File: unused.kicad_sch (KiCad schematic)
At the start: 7 parts, among them J6 FPGA GPIO, J7 FPGA_B3_GPIO, U8 T20Q144xx

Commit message: Added Manufacturer + Part info for most components.
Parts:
- C11, C14, C74, C75: Manufacturer (none) -> Samsung; Part (none) -> CL10B104KB8NFN
- J6: Manufacturer (none) -> Adam Tech; Part (none) -> PH2-20-UA
- J7: Manufacturer (none) -> Adam Tech; Part (none) -> PH2-08-UA
- U8: Manufacturer (none) -> Efinix; Part (none) -> T20Q144C4
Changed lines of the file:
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@@
+      (effects (font (size 1.27 1.27)) hide)
+    )
+    (property "Manufacturer" "Samsung" (at 88.9 97.79 0)
+      (effects (font (size 1.27 1.27)) hide)
+    )
+    (property "Part" "CL10B104KB8NFN" (at 88.9 97.79 0)
       (effects (font (size 1.27 1.27)) hide)
     )
@@
     )
     (property "Datasheet" "~" (at 86.36 173.99 0)
+      (effects (font (size 1.27 1.27)) hide)
+    )
+    (property "Manufacturer" "Adam Tech" (at 86.36 173.99 0)
+      (effects (font (size 1.27 1.27)) hide)
+    )
+    (property "Part" "PH2-08-UA" (at 86.36 173.99 0)
       (effects (font (size 1.27 1.27)) hide)
     )
@@
       (effects (font (size 1.27 1.27)) hide)
     )
+    (property "Manufacturer" "Samsung" (at 127 63.5 0)
+      (effects (font (size 1.27 1.27)) hide)
+    )
+    (property "Part" "CL10B104KB8NFN" (at 127 63.5 0)
+      (effects (font (size 1.27 1.27)) hide)
+    )
     (pin "1")
     (pin "2")
@@
     )
     (property "Datasheet" "~" (at 85.725 137.16 0)
+      (effects (font (size 1.27 1.27)) hide)
+    )
+    (property "Manufacturer" "Adam Tech" (at 85.725 137.16 0)
+      (effects (font (size 1.27 1.27)) hide)
+    )
+    (property "Part" "PH2-20-UA" (at 85.725 137.16 0)
       (effects (font (size 1.27 1.27)) hide)
     )
@@
     )
     (property "Datasheet" "https://www.efinixinc.com/docs/trion8-ds-v4.4.pdf" (at 194.31 152.4 0)
+      (effects (font (size 1.27 1.27)) hide)
+    )
+    (property "Manufacturer" "Efinix" (at 194.31 125.73 0)
+      (effects (font (size 1.27 1.27)) hide)
+    )
+    (property "Part" "T20Q144C4" (at 194.31 125.73 0)
       (effects (font (size 1.27 1.27)) hide)
     )
@@
       (effects (font (size 1.27 1.27)) hide)
     )
+    (property "Manufacturer" "Efinix" (at 191.77 76.2 0)
+      (effects (font (size 1.27 1.27)) hide)
+    )
+    (property "Part" "T20Q144C4" (at 191.77 76.2 0)
+      (effects (font (size 1.27 1.27)) hide)
+    )
     (pin "76")
     (pin "141")
@@
       (effects (font (size 1.27 1.27)) hide)
     )
+    (property "Manufacturer" "Samsung" (at 127 97.79 0)
+      (effects (font (size 1.27 1.27)) hide)
+    )
+    (property "Part" "CL10B104KB8NFN" (at 127 97.79 0)
+      (effects (font (size 1.27 1.27)) hide)
+    )
     (pin "1")
     (pin "2")
@@
       (effects (font (size 1.27 1.27)) hide)
     )
+    (property "Manufacturer" "Samsung" (at 105.41 98.425 0)
+      (effects (font (size 1.27 1.27)) hide)
+    )
+    (property "Part" "CL10B104KB8NFN" (at 105.41 98.425 0)
+      (effects (font (size 1.27 1.27)) hide)
+    )

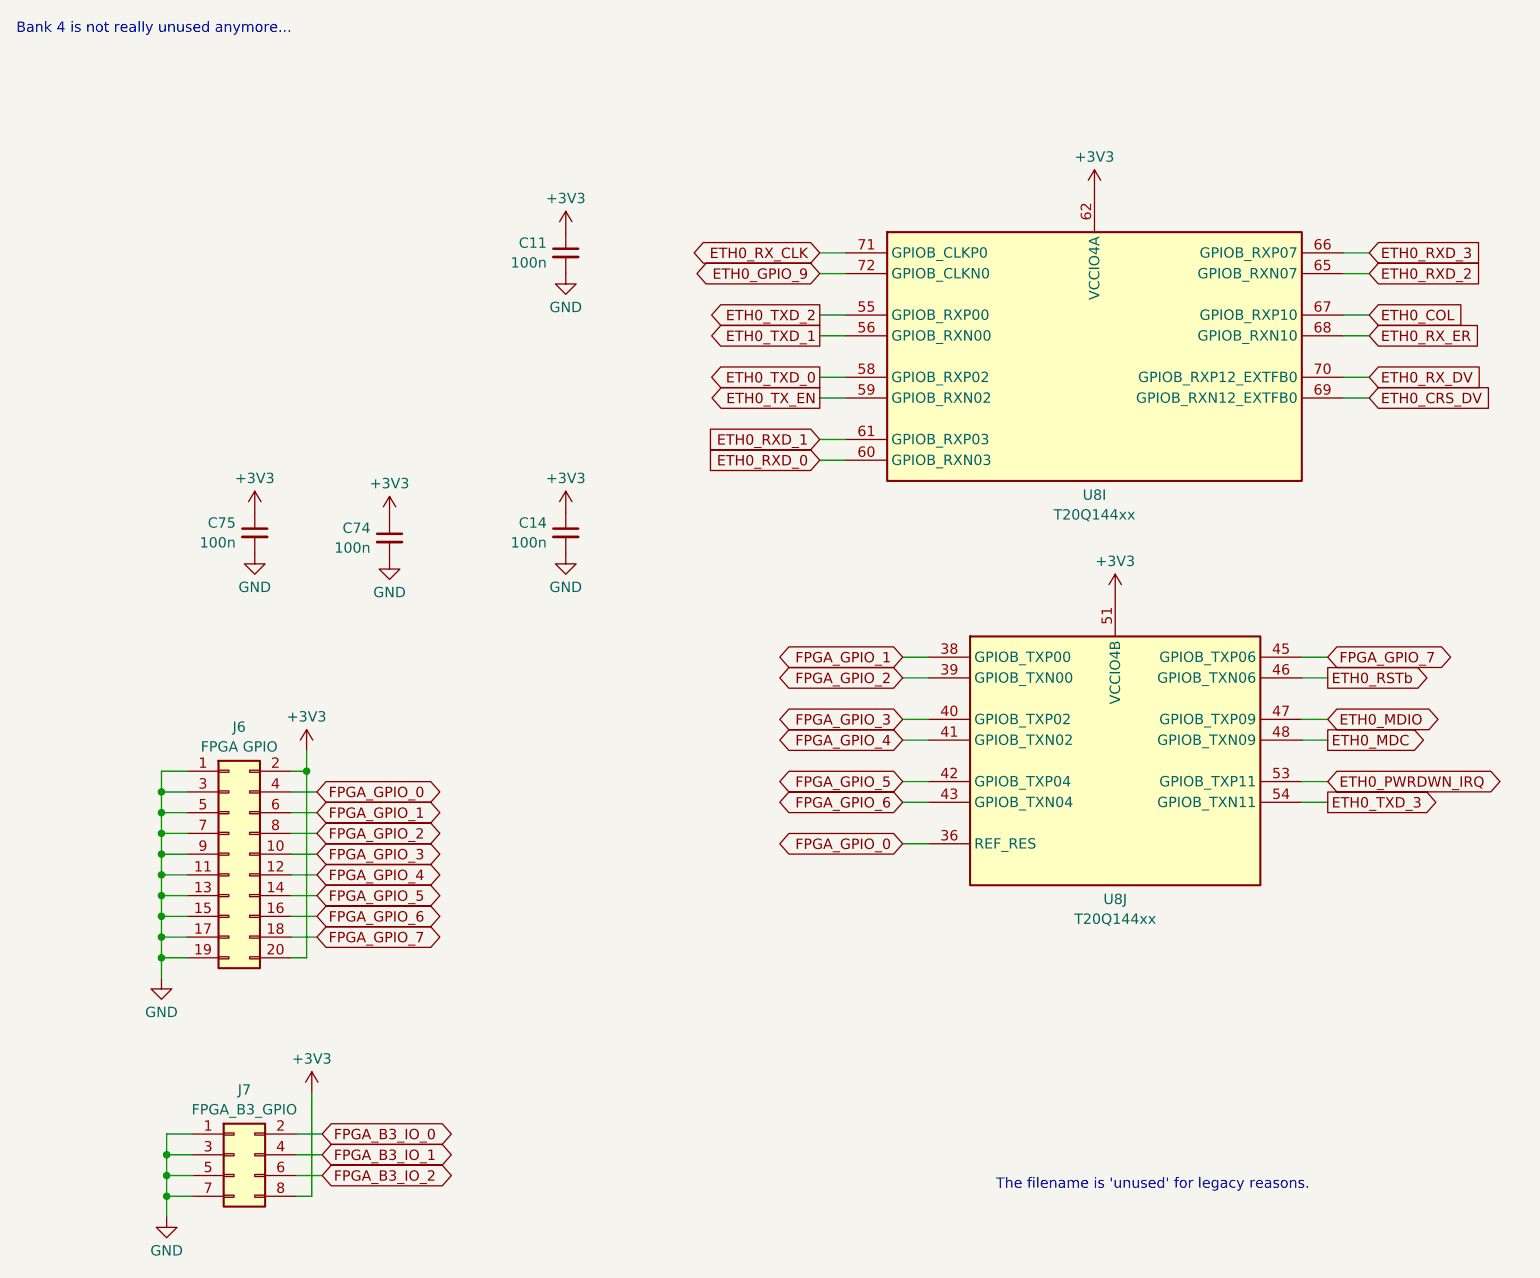
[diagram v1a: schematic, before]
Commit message: Added GPS receiver; increased board size
including battery supply; made board bigger
and added edge connectors for ETH GPIO, PPS
and antenna.
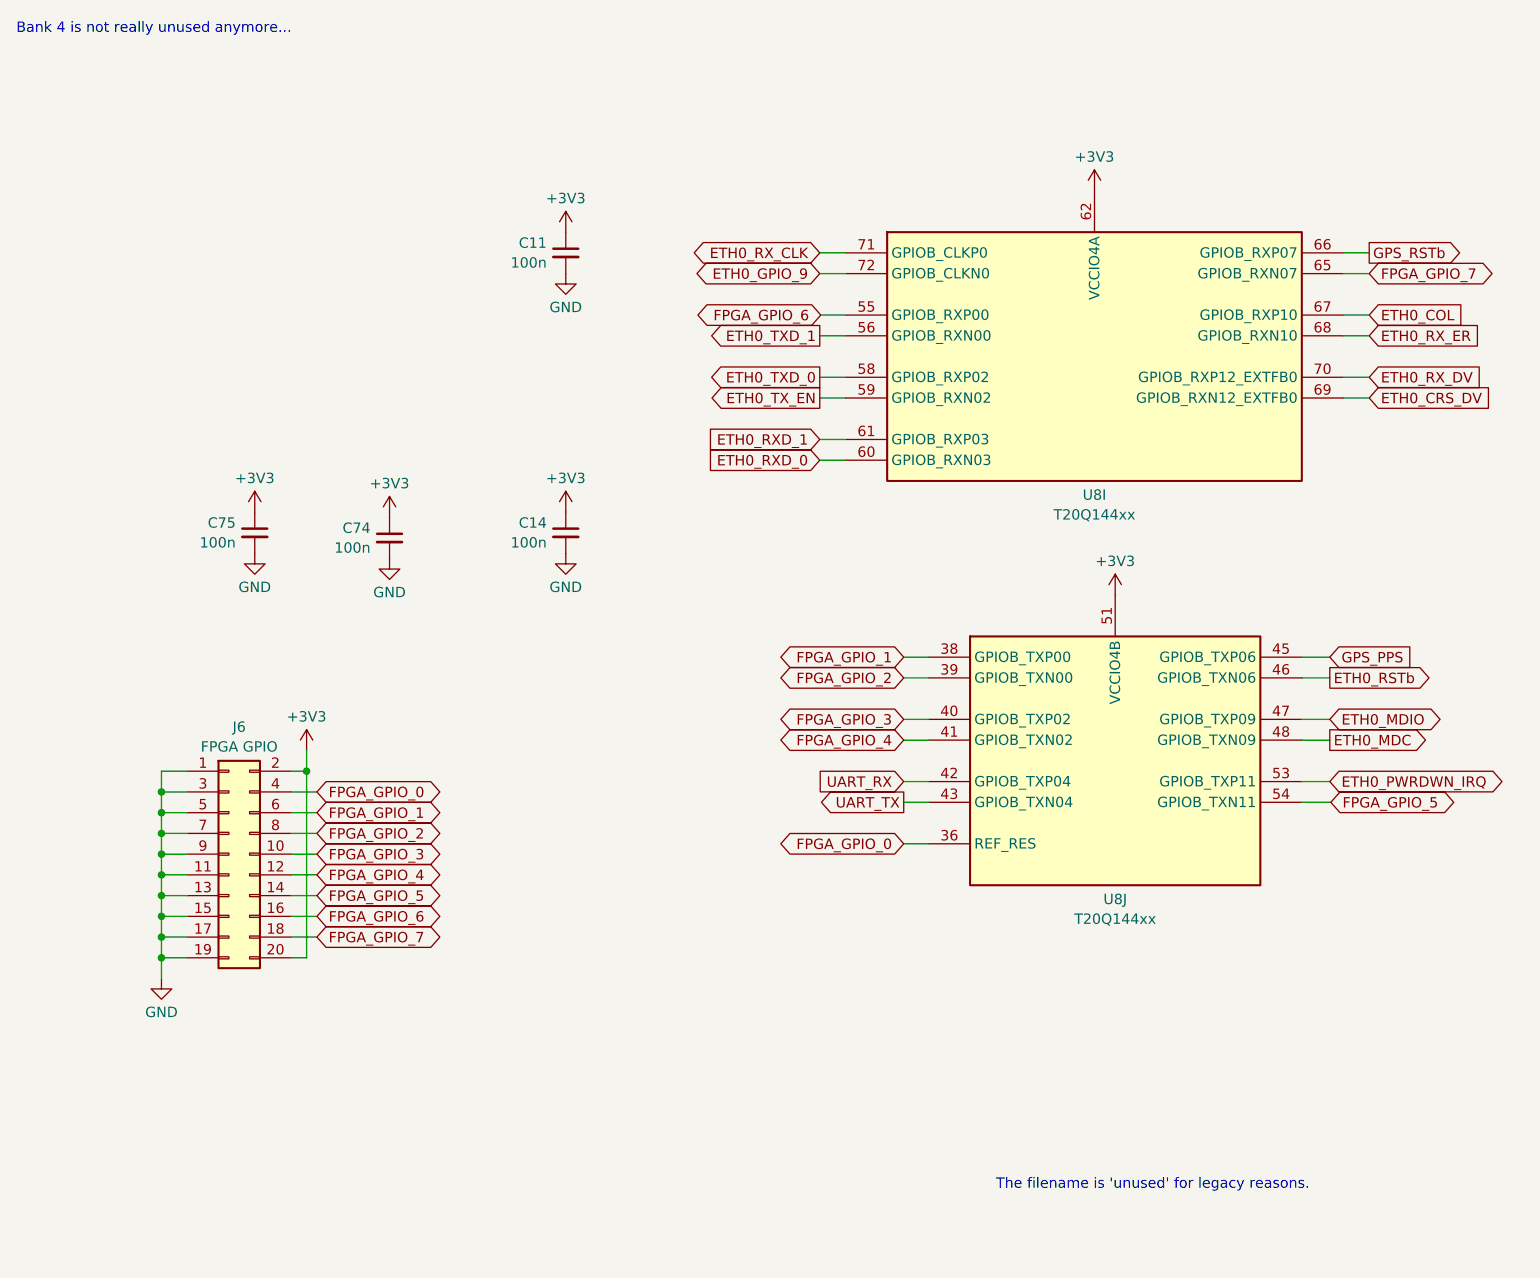
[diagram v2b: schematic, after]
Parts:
- removed J7: FPGA_B3_GPIO, Connector_PinHeader_2.54mm:PinHeader_2x04_P2.54mm_Vertical, symbol Connector_Generic:Conn_02x04_Odd_Even
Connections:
- net ETH0_RXD_2 is gone; now on net FPGA_GPIO_7: U8.65 (GPIOB_RXN07)
- net ETH0_TXD_2 is gone; now on net FPGA_GPIO_6: U8.55 (GPIOB_RXP00)
- net ETH0_TXD_3 is gone; now on net FPGA_GPIO_5: U8.54 (GPIOB_TXN11)
- net FPGA_GPIO_5: no longer U8.42 (GPIOB_TXP04)
- net FPGA_GPIO_6: no longer U8.43 (GPIOB_TXN04)
- net FPGA_GPIO_7: no longer U8.45 (GPIOB_TXP06)
- net ETH0_RXD_3 renamed GPS_RSTb
- new net GPS_PPS: U8.45 (GPIOB_TXP06)
- new net UART_RX: U8.42 (GPIOB_TXP04)
- new net UART_TX: U8.43 (GPIOB_TXN04)
